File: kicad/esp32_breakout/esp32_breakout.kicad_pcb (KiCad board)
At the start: 2 copper layers, 78 x 39 mm, 30 parts, among them J1 JST PH F, J10 JST PH F, J11 JST PH F, J2 JST PH F, J3 JST PH F, J4 DC-005 5.5x2.1mm, J5 Deans T-Plug M, J6 Header F, J7 Header F, J8 Header F, J9 JST PH F, Q1 BSS123, SW1 SS12D10, U1 ESP32 DEV KIT 30-pin, U2 Mini560-Pro

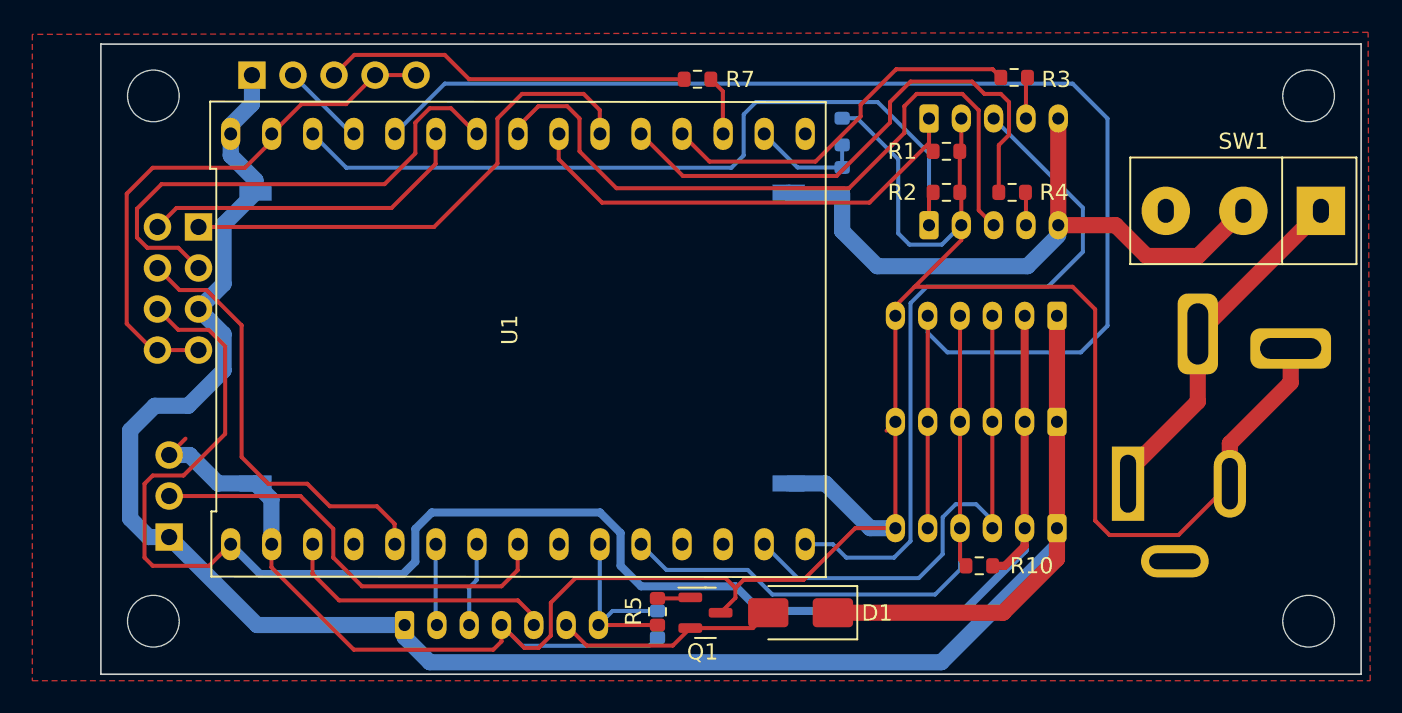
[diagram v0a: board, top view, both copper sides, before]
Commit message: ESP32 breakout v1.0
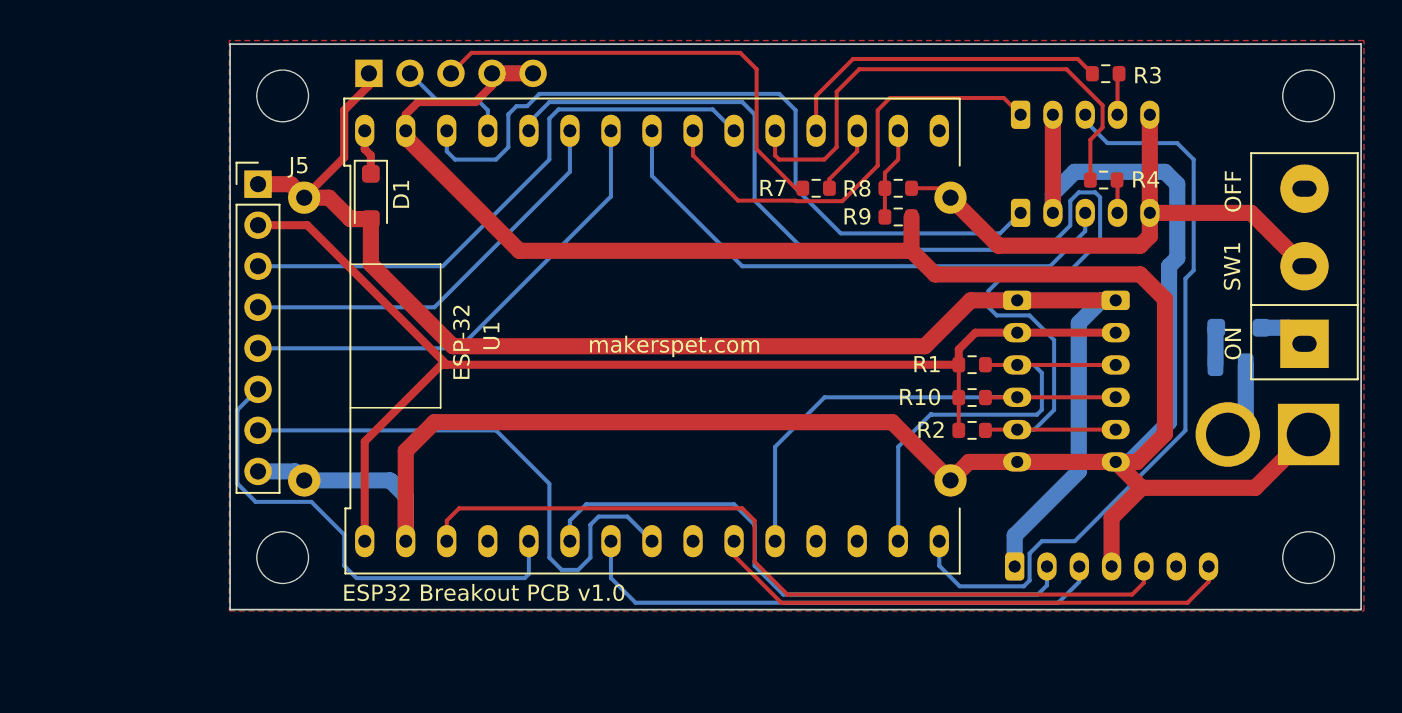
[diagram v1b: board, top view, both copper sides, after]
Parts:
- removed J11: JST PH F, Connector_JST:JST_PH_B6B-PH-K_1x06_P2.00mm_Vertical
- removed the J6 at (123.6, 89.5)
- removed J8: Header F, Connector_PinHeader_2.54mm:PinHeader_1x03_P2.54mm_Vertical
- removed Q1: BSS123, Package_TO_SOT_SMD:SOT-23
- removed R5: 1k, Resistor_SMD:R_0603_1608Metric
- removed R6: 10k, Resistor_SMD:R_0603_1608Metric
- added D2: FS26, Diode_SMD:D_SOD-123F, B.Cu at (188.0, 95.8)
- added F1: FCC20202AATP, Fuse:Fuse_0805_2012Metric, B.Cu at (187.5, 98.0)
- D1: value CGRA4004-G -> FS26; footprint Diode_SMD:D_SMA -> Diode_SMD:D_SOD-123F
- J1, J2: value JST PH F -> JST B5B-PH-K-S
- J10, J9: value JST PH F -> JST B6B-PH-K-S
- J3: value JST PH F -> JST B7B-PH-K-S
- J4: value DC-005 5.5x2.1mm -> J4; footprint Connector_BarrelJack:BarrelJack_GCT_DCJ200-10-A_Horizontal -> Makerspet:AMASS_XT30U-F_1x02_P5.0mm_Vertical
- J5: value Deans T-Plug M -> HDR F 2.54MM VERT; footprint Makerspet:DEANS-T-PLUG -> Connector_PinHeader_2.54mm:PinHeader_1x08_P2.54mm_Vertical; moved to F.Cu
- J6: renamed from J7; value Header F -> HDR F 2.54MM 5-pin VERT
- R10: value 4.7k -> 10k
- R8: moved to F.Cu
- R9: value 100k -> 10k; moved to F.Cu
- U1: value ESP32 DEV KIT 30-pin -> ESP32 DEV KIT Module 30-pin
- U2: value Mini560-Pro -> LM2596 Module; footprint Makerspet:Mini560-Pro -> Makerspet:LM2596 Module
- moved J5 61.8 mm to (127.3, 86.9), turned to 0 degrees
- moved J3 37.9 mm to (174.1, 110.5)
- moved D1 37.0 mm to (134.2, 87.6), turned to -90 degrees
- moved R2 14.8 mm to (171.4, 102.1)
- moved R1 13.3 mm to (171.4, 98.0)
- moved J4 11.6 mm to (192.3, 102.4), turned to 180 degrees
- moved R10 10.4 mm to (171.4, 100.1), turned to 0 degrees
- moved R7 9.97 mm to (161.8, 87.1)
- moved H4 8.92 mm to (128.8, 110.0)
- moved J10 8.35 mm to (180.3, 94.1), turned to -90 degrees
- moved U1 8.30 mm to (151.6, 96.3)
- moved H1 8.00 mm to (128.8, 81.4)
- moved J6 7.24 mm to (134.1, 80.0)
- moved U2 6.52 mm to (150.1, 96.5)
- moved R9 6.32 mm to (166.9, 88.9), turned to 180 degrees
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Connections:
- D1 pad 1: +5V -> Net-(D1-K)
- D1 pad 2: Net-(D1-A) -> +5V
- J3 pad 6: Net-(D1-A) -> unconnected-(J3-Pin_6-Pad6)
- J4 pad 1: +BATT -> GND
- J4 pad 2: GND -> Net-(J4-+)
- J5 pad 1: +BATT -> +5V
- J5 pad 2: GND -> +3V3
- R1 pad 1: /MOT_PWM_LEFT -> +3V3
- R1 pad 2: GND -> /I2C_SCL
- R2 pad 1: /MOT_PWM_RIGHT -> +3V3
- R2 pad 2: GND -> /I2C_INT
- SW1 pad 1: +BATT -> Net-(D2-K)
- U1 pad 30: +5V -> Net-(D1-K)
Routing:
- net +5V: track 129.3 -> 89.3 mm
- net /LDS_MOT_PWM: track 17.2 -> 49.7 mm
- net /LDS_TX: track 5.03 -> 36.4 mm
- net +3V3: track 103.6 -> 75.3 mm
- net /LDS_RX: track 5.22 -> 33.4 mm
- net +BATT: track 21.8 -> 0.00 mm
- net /LDS_MOT_EN: track 12.7 -> 32.9 mm
- net Net-(D1-A): track 13.9 -> 0.00 mm
- net /MOT_CW_RIGHT: track 44.1 -> 33.9 mm
- net /I2C_SDA: track 39.9 -> 30.2 mm
- net /I2C_INT: track 85.9 -> 77.8 mm
- net /GPIO5_BOOT_STRAP: track 26.9 -> 33.8 mm
- net +24V: track 41.3 -> 34.9 mm
- net GND: track 201.9 -> 195.7 mm
- net Net-(J6-Pin_3): track 22.8 -> 28.7 mm
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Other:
- board size 78 x 39 mm -> 70 x 35 mm
- board text added: "BATT"
- board text added: "DIST"
- board text added: "ESP32 Breakout PCB v1.0"
- board text added: "EXT"
- board text added: "LEFT"
- board text added: "LM2596 DC-DC Module"
- board text added: "MOTORS"
- board text added: "OFF"
- board text added: "ON"
- board text added: "RIGHT"
- board text added: "makerspet.com"
